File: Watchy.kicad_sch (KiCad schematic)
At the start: 73 parts, among them J1 FPC24(0.5MM), J2 USB_C_Receptacle_USB2.0, J3 Battery, M1 Vibration_Motor, Q1 AO3400A, Q2 UMH3N, Q4 CJ2301, Q5 S8050, SW1 BTN, SW2 BTN, SW3 BTN, SW4 BTN, U1 ESP32-PICO-D4, U2 ME6211C33M5G-N, U3 CP2102, U4 BMA423, U5 TP4054, U6 PCF8563BS, Y1 32.768KHz

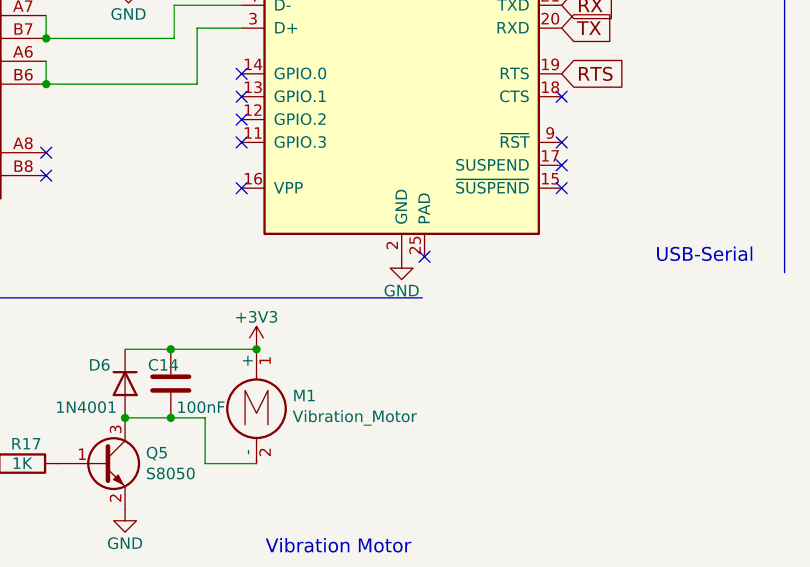
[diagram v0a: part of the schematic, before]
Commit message: Gerbers erstellt
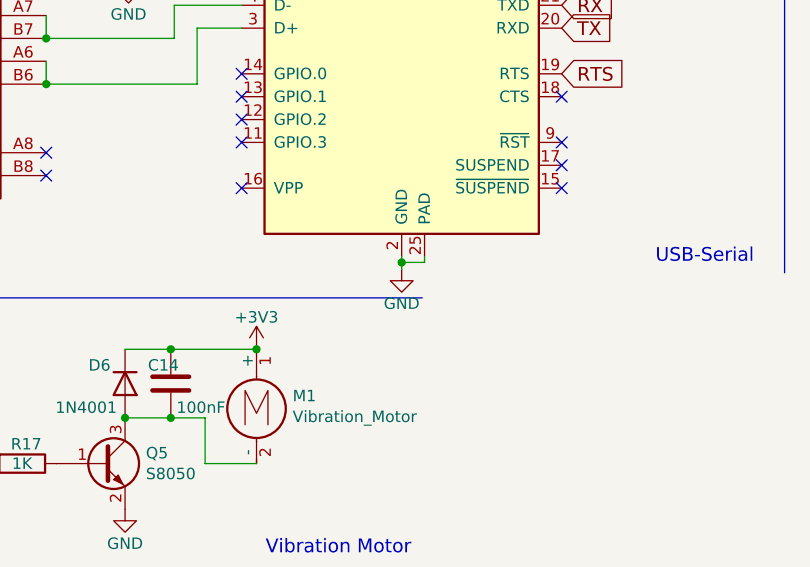
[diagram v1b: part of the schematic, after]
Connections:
- net GND: now also U3.25 (PAD)
- no-connect marks 35 -> 34
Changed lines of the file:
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@@
   (junction (at 134.366 145.034) (diameter 0) (color 0 0 0 0)
+  )
+  (junction (at 173.863 164.846) (diameter 0) (color 0 0 0 0)
   )
   (junction (at 173.863 115.951) (diameter 0) (color 0 0 0 0)
@@
   (no_connect (at 156.083 146.431))
   (no_connect (at 191.643 131.191))
-  (no_connect (at 176.403 164.211))
   (no_connect (at 245.618 39.497))
   (no_connect (at 156.083 151.511))
@@
     (stroke (width 0) (type default))
   )
+  (wire (pts (xy 173.863 164.846) (xy 173.863 164.211))
+    (stroke (width 0) (type default))
+  )
   (wire (pts (xy 152.019 182.118) (xy 152.019 187.198))
     (stroke (width 0) (type default))
@@
     (stroke (width 0) (type default))
   )
+  (wire (pts (xy 176.403 164.211) (xy 176.403 164.846))
+    (stroke (width 0) (type default))
+  )
   (wire (pts (xy 134.366 142.494) (xy 134.366 145.034))
     (stroke (width 0) (type default))
@@
     (stroke (width 0) (type default))
   )
+  (wire (pts (xy 176.403 164.846) (xy 173.863 164.846))
+    (stroke (width 0) (type default))
+  )
   (wire (pts (xy 143.51 132.334) (xy 143.51 133.477))
     (stroke (width 0) (type default))
@@
   )
   (polyline (pts (xy 83.058 168.783) (xy 83.058 197.993))
+    (stroke (width 0) (type default))
+  )
+  (wire (pts (xy 173.863 165.608) (xy 173.863 164.846))
     (stroke (width 0) (type default))
   )
@@
     )
   )
-  (symbol (lib_id "power:GND") (at 173.863 164.211 0) (unit 1)
-    (in_bom yes) (on_board yes) (dnp no)
-    (property "Reference" "#PWR060" (at 173.863 170.561 0)
-      (effects (font (size 1.27 1.27)) hide)
-    )
-    (property "Value" "GND" (at 173.863 168.021 0)
-      (effects (font (size 1.27 1.27)))
-    )
-    (property "Footprint" "" (at 173.863 164.211 0)
-      (effects (font (size 1.27 1.27)) hide)
-    )
-    (property "Datasheet" "" (at 173.863 164.211 0)
-      (effects (font (size 1.27 1.27)) hide)
-    )
+  (symbol (lib_id "power:GND") (at 173.863 165.608 0) (unit 1)
+    (in_bom yes) (on_board yes) (dnp no)
+    (property "Reference" "#PWR060" (at 173.863 171.958 0)
+      (effects (font (size 1.27 1.27)) hide)
+    )
+    (property "Value" "GND" (at 173.863 169.418 0)
+      (effects (font (size 1.27 1.27)))
+    )
+    (property "Footprint" "" (at 173.863 165.608 0)
+      (effects (font (size 1.27 1.27)) hide)
+    )
+    (property "Datasheet" "" (at 173.863 165.608 0)
+      (effects (font (size 1.27 1.27)) hide)
+    )
